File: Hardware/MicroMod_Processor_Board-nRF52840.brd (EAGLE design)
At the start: 22 x 22 mm, 30 parts, among them J2 MICROMOD-2222, U1 W25QXX128MBIT-6X5, U2 MDBT50Q, Y1 32.768kHz

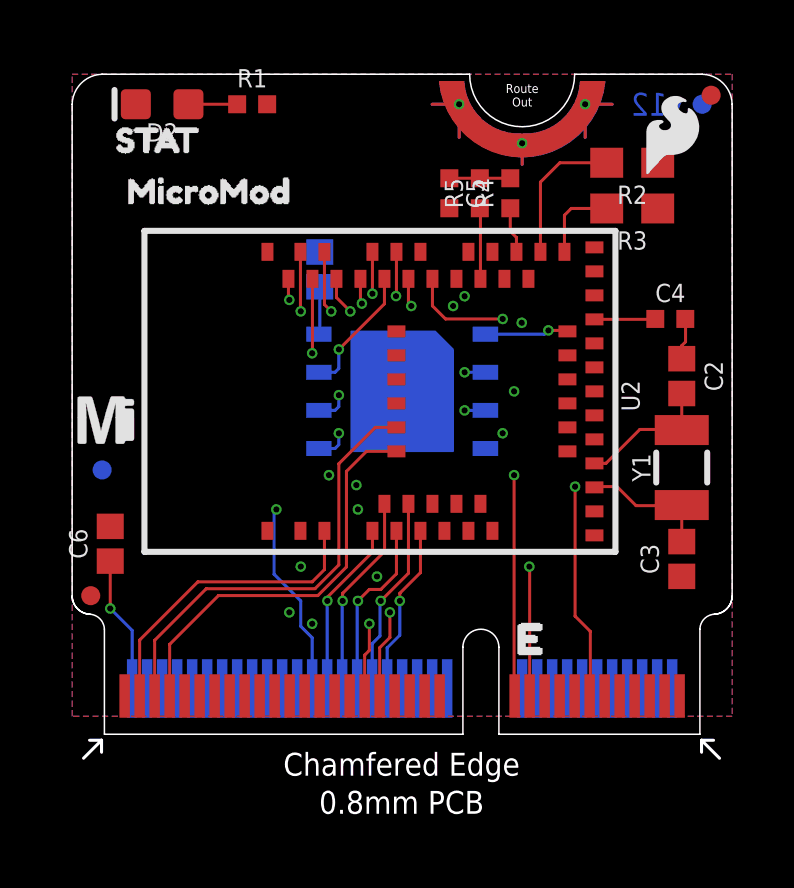
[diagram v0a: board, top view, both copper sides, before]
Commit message: Update MicroMod_Processor_Board-nRF52840.brd
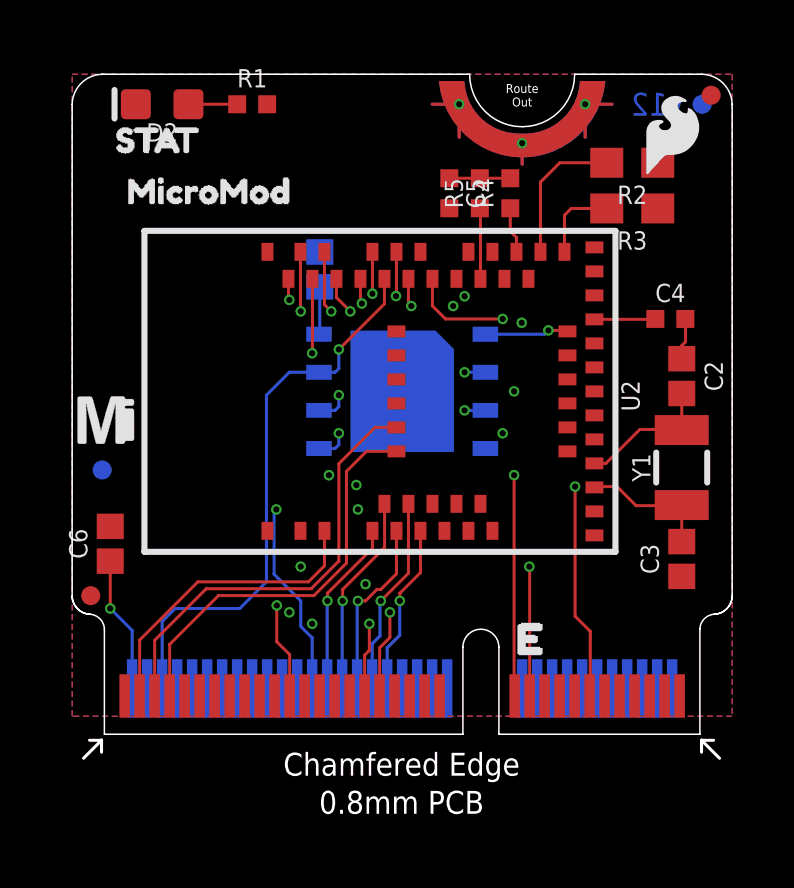
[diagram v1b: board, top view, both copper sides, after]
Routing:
- net SPI_!CS!: track 4.34 -> 18.9 mm
- net SCL1: track 10.9 -> 17.6 mm, vias 2 -> 3
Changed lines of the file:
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@@
 <layer number="37" name="tTest" color="7" fill="1" visible="no" active="yes"/>
 <layer number="38" name="bTest" color="7" fill="1" visible="no" active="yes"/>
-<layer number="39" name="tKeepout" color="4" fill="11" visible="no" active="yes"/>
+<layer number="39" name="tKeepout" color="4" fill="11" visible="yes" active="yes"/>
 <layer number="40" name="bKeepout" color="1" fill="11" visible="no" active="yes"/>
 <layer number="41" name="tRestrict" color="4" fill="10" visible="no" active="yes"/>
@@
 <wire x1="8.89" y1="12.192" x2="8.763" y2="12.065" width="0.1016" layer="16"/>
 <wire x1="8.763" y1="12.065" x2="8.225" y2="12.065" width="0.1016" layer="16"/>
-<wire x1="3" y1="1.525" x2="8.225" y2="12.065" width="0" layer="19" extent="16-16"/>
+<wire x1="8.225" y1="12.065" x2="7.239" y2="12.065" width="0.1016" layer="16"/>
+<wire x1="7.239" y1="12.065" x2="6.477" y2="11.303" width="0.1016" layer="16"/>
+<wire x1="6.477" y1="5.08" x2="5.588" y2="4.191" width="0.1016" layer="16"/>
+<wire x1="5.588" y1="4.191" x2="3.429" y2="4.191" width="0.1016" layer="16"/>
+<wire x1="3.429" y1="4.191" x2="3" y2="3.762" width="0.1016" layer="16"/>
+<wire x1="3" y1="3.762" x2="3" y2="1.525" width="0.1016" layer="16"/>
+<wire x1="6.477" y1="11.303" x2="6.477" y2="5.08" width="0.1016" layer="16"/>
 </signal>
 <signal name="LED_BUILTIN">
@@
 <contactref element="U2" pad="3"/>
 <wire x1="2.25" y1="1.275" x2="2.25" y2="3.139" width="0.1016" layer="1"/>
-<wire x1="8.41" y1="5.489" x2="8.41" y2="6.78" width="0.1016" layer="1"/>
+<wire x1="8.41" y1="6.78" x2="8.41" y2="5.616" width="0.1016" layer="1"/>
 <wire x1="2.25" y1="3.139" x2="4.191" y2="5.08" width="0.1016" layer="1"/>
-<wire x1="4.191" y1="5.08" x2="8.001" y2="5.08" width="0.1016" layer="1"/>
-<wire x1="8.001" y1="5.08" x2="8.41" y2="5.489" width="0.1016" layer="1"/>
+<wire x1="4.191" y1="5.08" x2="7.874" y2="5.08" width="0.1016" layer="1"/>
+<wire x1="7.874" y1="5.08" x2="8.41" y2="5.616" width="0.1016" layer="1"/>
 </signal>
 <signal name="GPIO7">
@@
 <contactref element="U2" pad="56"/>
 <wire x1="3.25" y1="1.275" x2="3.25" y2="2.996" width="0.1016" layer="1"/>
-<wire x1="8.1903875" y1="4.6228" x2="9.144" y2="5.5764125" width="0.1016" layer="1"/>
+<wire x1="8.0633875" y1="4.6228" x2="9.144" y2="5.7034125" width="0.1016" layer="1"/>
 <wire x1="9.811" y1="9.43" x2="10.81" y2="9.43" width="0.1016" layer="1"/>
 <wire x1="3.25" y1="2.996" x2="4.8768" y2="4.6228" width="0.1016" layer="1"/>
-<wire x1="4.8768" y1="4.6228" x2="8.1903875" y2="4.6228" width="0.1016" layer="1"/>
-<wire x1="9.144" y1="5.5764125" x2="9.144" y2="8.763" width="0.1016" layer="1"/>
+<wire x1="4.8768" y1="4.6228" x2="8.0633875" y2="4.6228" width="0.1016" layer="1"/>
+<wire x1="9.144" y1="5.7034125" x2="9.144" y2="8.763" width="0.1016" layer="1"/>
 <wire x1="9.144" y1="8.763" x2="9.811" y2="9.43" width="0.1016" layer="1"/>
 </signal>
@@
 <contactref element="U2" pad="57"/>
 <wire x1="2.75" y1="1.275" x2="2.75" y2="3.131" width="0.1016" layer="1"/>
-<wire x1="4.4704" y1="4.8514" x2="8.09569375" y2="4.8514" width="0.1016" layer="1"/>
-<wire x1="8.09569375" y1="4.8514" x2="8.89" y2="5.64570625" width="0.1016" layer="1"/>
-<wire x1="8.89" y1="5.64570625" x2="8.89" y2="9.017" width="0.1016" layer="1"/>
+<wire x1="4.4704" y1="4.8514" x2="7.96869375" y2="4.8514" width="0.1016" layer="1"/>
+<wire x1="7.96869375" y1="4.8514" x2="8.89" y2="5.77270625" width="0.1016" layer="1"/>
+<wire x1="8.89" y1="5.77270625" x2="8.89" y2="9.017" width="0.1016" layer="1"/>
 <wire x1="8.89" y1="9.017" x2="10.103" y2="10.23" width="0.1016" layer="1"/>
 <wire x1="10.103" y1="10.23" x2="10.81" y2="10.23" width="0.1016" layer="1"/>
@@
 <wire x1="9" y1="4.428" x2="9.017" y2="4.445" width="0.1016" layer="16"/>
 <via x="9.017" y="4.445" extent="1-16" drill="0.2032"/>
-<wire x1="10.414" y1="6.096" x2="9.017" y2="4.699" width="0.1016" layer="1"/>
-<wire x1="9.017" y1="4.445" x2="9.017" y2="4.699" width="0.1016" layer="1"/>
-<wire x1="10.414" y1="6.096" x2="10.414" y2="7.676" width="0.1016" layer="1"/>
+<wire x1="10.414" y1="6.223" x2="9.017" y2="4.826" width="0.1016" layer="1"/>
+<wire x1="9.017" y1="4.445" x2="9.017" y2="4.826" width="0.1016" layer="1"/>
+<wire x1="10.414" y1="6.223" x2="10.414" y2="7.676" width="0.1016" layer="1"/>
 <wire x1="10.414" y1="7.676" x2="10.41" y2="7.68" width="0.1016" layer="1"/>
 </signal>
@@
 <via x="9.525" y="4.445" extent="1-16" drill="0.2032"/>
 <wire x1="10.81" y1="5.349" x2="10.81" y2="6.78" width="0.1016" layer="1"/>
-<wire x1="9.525" y1="4.445" x2="9.906" y2="4.826" width="0.1016" layer="1"/>
-<wire x1="10.287" y1="4.826" x2="9.906" y2="4.826" width="0.1016" layer="1"/>
+<wire x1="10.16" y1="4.826" x2="9.779" y2="4.445" width="0.1016" layer="1"/>
+<wire x1="9.525" y1="4.445" x2="9.779" y2="4.445" width="0.1016" layer="1"/>
+<wire x1="10.287" y1="4.826" x2="10.16" y2="4.826" width="0.1016" layer="1"/>
 <wire x1="10.81" y1="5.349" x2="10.287" y2="4.826" width="0.1016" layer="1"/>
 </signal>
@@
 <wire x1="8.5" y1="4.436" x2="8.509" y2="4.445" width="0.1016" layer="16"/>
 <via x="8.509" y="4.445" extent="1-16" drill="0.2032"/>
-<wire x1="10.01" y1="6.073" x2="10.01" y2="6.78" width="0.1016" layer="1"/>
-<wire x1="8.509" y1="4.445" x2="8.509" y2="4.572" width="0.1016" layer="1"/>
-<wire x1="10.01" y1="6.073" x2="8.509" y2="4.572" width="0.1016" layer="1"/>
+<wire x1="10.01" y1="6.2" x2="10.01" y2="6.78" width="0.1016" layer="1"/>
+<wire x1="8.509" y1="4.445" x2="8.509" y2="4.699" width="0.1016" layer="1"/>
+<wire x1="10.01" y1="6.2" x2="8.509" y2="4.699" width="0.1016" layer="1"/>
 </signal>
 <signal name="GPIO0">
@@
 <wire x1="10.01" y1="16.08" x2="10.01" y2="14.68486875" width="0.1016" layer="1"/>
 <via x="10.01" y="14.68486875" extent="1-16" drill="0.2032"/>
-<wire x1="10.01" y1="14.68486875" x2="10.01" y2="7.62" width="0.1016" layer="15"/>
-<wire x1="10.01" y1="7.62" x2="10.01" y2="7.47" width="0.1016" layer="15"/>
-<wire x1="10.01" y1="7.47" x2="10.01" y2="5.4078" width="0.1016" layer="15"/>
-<wire x1="10.01" y1="5.4078" x2="10.16" y2="5.2578" width="0.1016" layer="15"/>
-<via x="10.16" y="5.2578" extent="1-16" drill="0.2032"/>
-<wire x1="7.25" y1="1.275" x2="10.16" y2="5.2578" width="0" layer="19" extent="1-1"/>
+<wire x1="10.01" y1="14.68486875" x2="10.01" y2="5.2348" width="0.1016" layer="15"/>
+<wire x1="10.01" y1="5.2348" x2="9.779" y2="5.0038" width="0.1016" layer="15"/>
+<via x="9.779" y="5.0038" extent="1-16" drill="0.2032"/>
+<wire x1="9.779" y1="5.0038" x2="7.53221875" y2="5.0038" width="0.1016" layer="2"/>
+<wire x1="7.53221875" y1="5.0038" x2="6.82101875" y2="4.2926" width="0.1016" layer="2"/>
+<via x="6.82101875" y="4.2926" extent="1-16" drill="0.2032"/>
+<wire x1="6.82101875" y1="4.2926" x2="6.82101875" y2="3.08498125" width="0.1016" layer="1"/>
+<wire x1="7.25" y1="2.656" x2="7.25" y2="1.275" width="0.1016" layer="1"/>
+<wire x1="6.82101875" y1="3.08498125" x2="7.25" y2="2.656" width="0.1016" layer="1"/>
 </signal>
 <signal name="SDA1">
